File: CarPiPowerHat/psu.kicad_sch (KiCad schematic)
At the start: 38 parts, among them IC2 BD2226G-TR, J7 USB_A, J8 Conn_01x02_Male, Q4 DMP3013SFV-7, U3 AP64501SP-13

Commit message: Finalized 2.2
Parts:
- IC2: LCSC C308587Copy -> C308587
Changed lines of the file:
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@@
       (effects (font (size 1.27 1.27)) (justify left) hide)
     )
-    (property "LCSC" "C308587Copy" (id 12) (at 73.66 156.21 0)
+    (property "LCSC" "C308587" (id 12) (at 73.66 156.21 0)
       (effects (font (size 1.27 1.27)) hide)
     )

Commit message: Finalizing, checking parts
Might be ready for production
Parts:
- C38: footprint Capacitor_SMD:C_0603_1608Metric_Pad1.08x0.95mm_HandSolder -> Capacitor_SMD:C_1206_3216Metric_Pad1.33x1.80mm_HandSolder; LCSC (none) -> C15008
- C39: LCSC (none) -> C15849
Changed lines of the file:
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@@
       (effects (font (size 1.27 1.27)) (justify left))
     )
-    (property "Footprint" "Capacitor_SMD:C_0603_1608Metric_Pad1.08x0.95mm_HandSolder" (id 2) (at 51.7652 165.1 0)
+    (property "Footprint" "Capacitor_SMD:C_1206_3216Metric_Pad1.33x1.80mm_HandSolder" (id 2) (at 51.7652 165.1 0)
       (effects (font (size 1.27 1.27)) hide)
     )
@@
     )
     (property "Field4" "low ESR" (id 4) (at 50.8 161.29 0)
+      (effects (font (size 1.27 1.27)) hide)
+    )
+    (property "LCSC" "C15008" (id 5) (at 50.8 161.29 0)
       (effects (font (size 1.27 1.27)) hide)
     )
@@
       (effects (font (size 1.27 1.27)) hide)
     )
+    (property "LCSC" "C15849" (id 4) (at 60.325 161.29 0)
+      (effects (font (size 1.27 1.27)) hide)
+    )

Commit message: Moved HDMI ports
The HDMI ports were offset by 1-2 mm
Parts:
- C10, C14, C15, C17, C18, C19, C8: LCSC C162422 -> C440198
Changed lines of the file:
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@@
       (effects (font (size 1.27 1.27)) hide)
     )
-    (property "LCSC" "C162422" (id 10) (at 41.783 116.078 0)
+    (property "LCSC" "C440198" (id 10) (at 41.783 116.078 0)
       (effects (font (size 1.27 1.27)) hide)
     )
@@
       (effects (font (size 1.27 1.27)) hide)
     )
-    (property "LCSC" "C162422" (id 10) (at 52.578 116.078 0)
+    (property "LCSC" "C440198" (id 10) (at 52.578 116.078 0)
       (effects (font (size 1.27 1.27)) hide)
     )
@@
       (effects (font (size 1.27 1.27)) hide)
     )
-    (property "LCSC" "C162422" (id 10) (at 63.373 116.078 0)
+    (property "LCSC" "C440198" (id 10) (at 63.373 116.078 0)
       (effects (font (size 1.27 1.27)) hide)
     )
@@
       (effects (font (size 1.27 1.27)) hide)
     )
-    (property "LCSC" "C162422" (id 10) (at 73.533 116.078 0)
+    (property "LCSC" "C440198" (id 10) (at 73.533 116.078 0)
       (effects (font (size 1.27 1.27)) hide)
     )
@@
       (effects (font (size 1.27 1.27)) hide)
     )
-    (property "LCSC" "C162422" (id 10) (at 84.328 116.078 0)
+    (property "LCSC" "C440198" (id 10) (at 84.328 116.078 0)
       (effects (font (size 1.27 1.27)) hide)
     )
@@
       (effects (font (size 1.27 1.27)) hide)
     )
-    (property "LCSC" "C162422" (id 10) (at 95.758 116.078 0)
+    (property "LCSC" "C440198" (id 10) (at 95.758 116.078 0)
       (effects (font (size 1.27 1.27)) hide)
     )
@@
       (effects (font (size 1.27 1.27)) hide)
     )
-    (property "LCSC" "C162422" (id 10) (at 125.73 44.45 0)
-      (effects (font (size 1.27 1.27)) hide)
-    )
+    (property "LCSC" "C440198" (id 10) (at 125.73 44.45 0)
+      (effects (font (size 1.27 1.27)) hide)
+    )

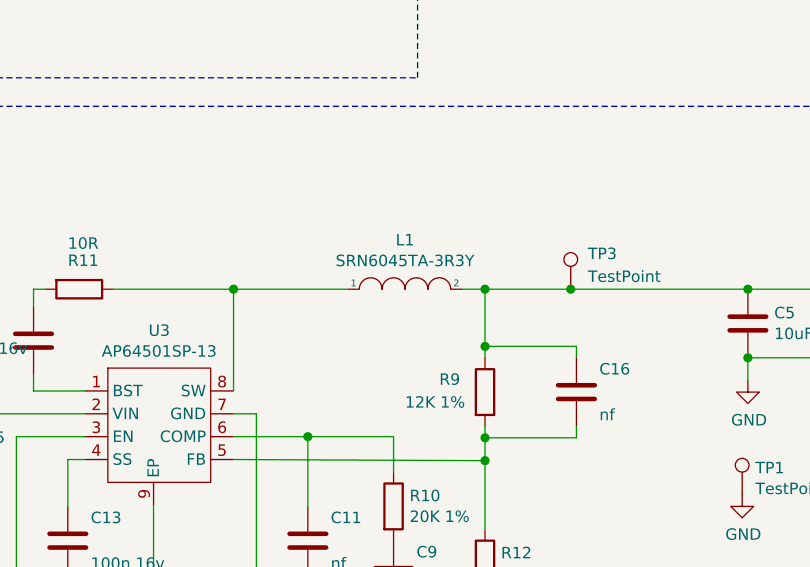
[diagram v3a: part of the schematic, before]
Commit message: Some bugfixing, added cam.py script
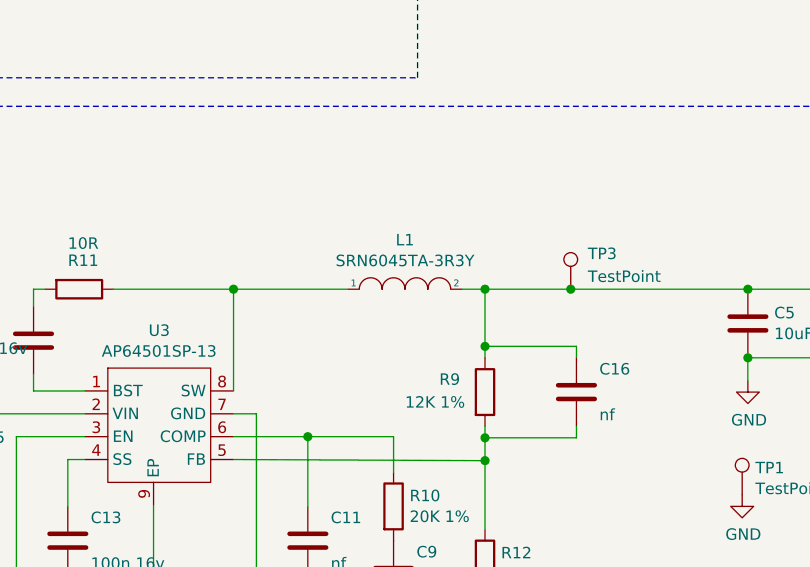
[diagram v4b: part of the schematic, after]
